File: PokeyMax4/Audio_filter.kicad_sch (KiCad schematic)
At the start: 16 parts, among them U1 TSV854IQ4T

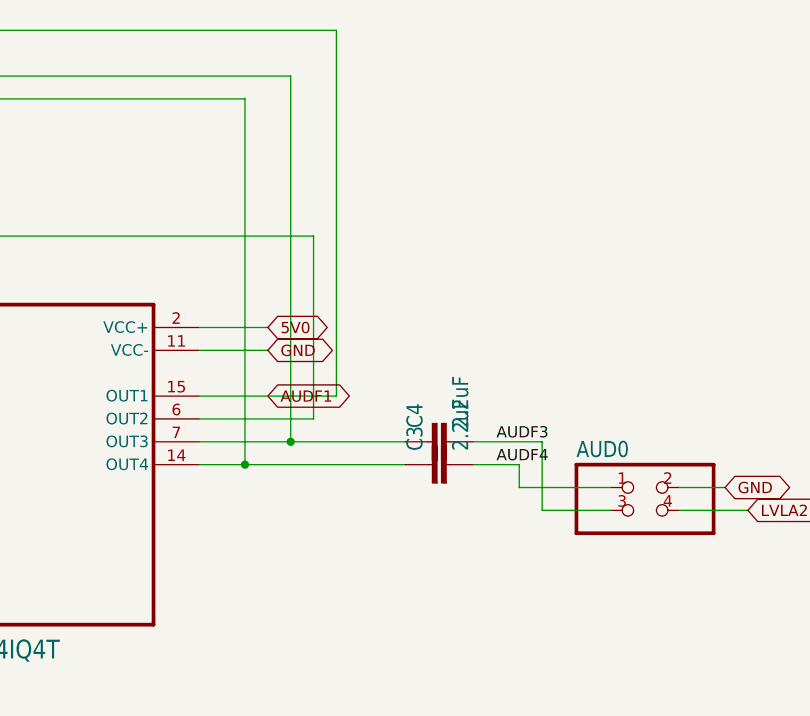
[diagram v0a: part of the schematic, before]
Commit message: Final adjustements to production files for JLC
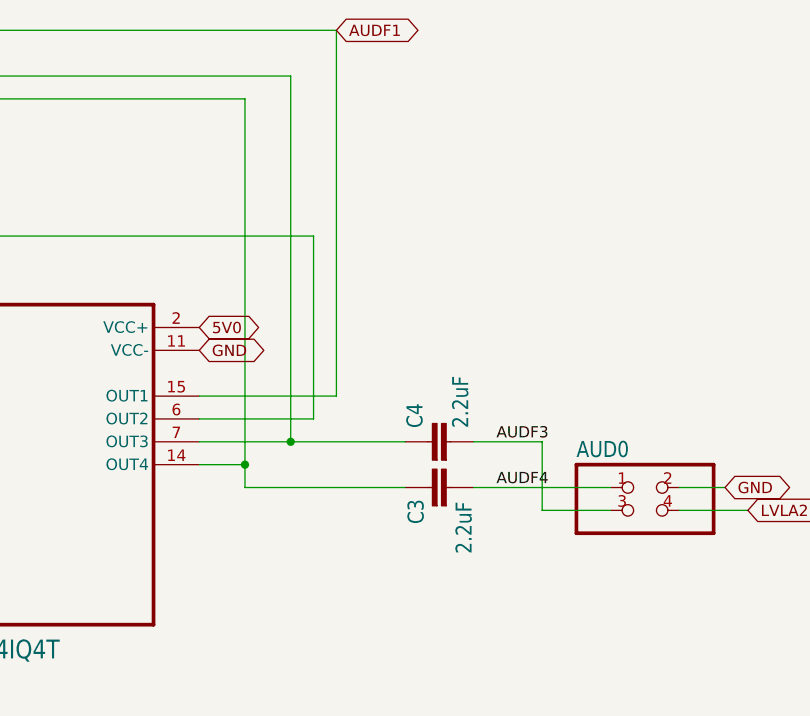
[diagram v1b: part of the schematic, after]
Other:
- moved on the sheet: C3
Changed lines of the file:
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@@
+	(wire
+		(pts
+			(xy 185.42 104.14) (xy 185.42 101.6)
+		)
+		(stroke
+			(width 0.1524)
+			(type solid)
+		)
+	)
 	(wire
 		(pts
@@
 	(wire
 		(pts
-			(xy 185.42 101.6) (xy 203.2 101.6)
+			(xy 185.42 104.14) (xy 203.2 104.14)
 		)
 		(stroke
@@
 	(wire
 		(pts
-			(xy 226.06 104.14) (xy 215.9 104.14)
-		)
-		(stroke
-			(width 0.1524)
-			(type solid)
-		)
-	)
-	(wire
-		(pts
 			(xy 68.58 99.06) (xy 68.58 109.22)
 		)
@@
 	(wire
 		(pts
-			(xy 180.34 88.9) (xy 187.96 88.9)
-		)
-		(stroke
-			(width 0.1524)
-			(type solid)
-		)
-	)
-	(wire
-		(pts
 			(xy 132.08 152.4) (xy 111.76 152.4)
 		)
@@
 	(wire
 		(pts
-			(xy 215.9 101.6) (xy 210.82 101.6)
+			(xy 210.82 104.14) (xy 226.06 104.14)
 		)
 		(stroke
@@
 	(wire
 		(pts
-			(xy 187.96 86.36) (xy 180.34 86.36)
-		)
-		(stroke
-			(width 0.1524)
-			(type solid)
-		)
-	)
-	(wire
-		(pts
 			(xy 101.6 142.24) (xy 132.08 142.24)
 		)
@@
 	(wire
 		(pts
-			(xy 215.9 104.14) (xy 215.9 101.6)
-		)
-		(stroke
-			(width 0.1524)
-			(type solid)
-		)
-	)
-	(wire
-		(pts
 			(xy 190.5 99.06) (xy 190.5 58.42)
 		)
@@
 	)
 	(label "AUDF4"
-		(at 213.36 101.6 0)
+		(at 213.36 104.14 0)
 		(fields_autoplaced yes)
 		(effects
@@
 	(global_label "5V0"
 		(shape bidirectional)
-		(at 187.96 86.36 0)
+		(at 180.34 86.36 0)
 		(fields_autoplaced yes)
 		(effects
@@
 		)
 		(property "Intersheetrefs" "${INTERSHEET_REFS}"
-			(at 195.4116 86.36 0)
+			(at 187.7916 86.36 0)
 			(effects
 				(font
@@
 	(global_label "GND"
 		(shape bidirectional)
-		(at 187.96 88.9 0)
+		(at 180.34 88.9 0)
 		(fields_autoplaced yes)
 		(effects
@@
 		)
 		(property "Intersheetrefs" "${INTERSHEET_REFS}"
-			(at 195.7673 88.9 0)
+			(at 188.1473 88.9 0)
 			(effects
 				(font
@@
 	(global_label "AUDF1"
 		(shape bidirectional)
-		(at 187.96 93.98 0)
+		(at 195.58 53.34 0)
 		(fields_autoplaced yes)
 		(effects
@@
 		)
 		(property "Intersheetrefs" "${INTERSHEET_REFS}"
-			(at 197.8416 93.98 0)
+			(at 205.4616 53.34 0)
 			(effects
 				(font
@@
 	(symbol
 		(lib_id "pokeymax4-eagle-import:C-EUC0402")
-		(at 205.74 101.6 90)
+		(at 205.74 104.14 90)
 		(unit 1)
 		(exclude_from_sim no)
@@
 		(dnp no)
 		(property "Reference" "C3"
-			(at 205.359 100.076 0)
+			(at 205.486 108.204 0)
 			(effects
 				(font
@@
 		)
 		(property "Value" "2.2uF"
-			(at 210.439 100.076 0)
+			(at 210.82 111.506 0)
 			(effects
 				(font
@@
 		)
 		(property "Footprint" "pokeymax4:C0402"
-			(at 205.74 101.6 0)
+			(at 205.74 104.14 0)
 			(effects
 				(font
@@
 		)
 		(property "Datasheet" ""
-			(at 205.74 101.6 0)
+			(at 205.74 104.14 0)
 			(effects
 				(font
@@
 		)
 		(property "Description" ""
-			(at 205.74 101.6 0)
+			(at 205.74 104.14 0)
 			(effects
 				(font
@@
 		)
 		(property "LCSC Part #" "C12530"
-			(at 205.74 101.6 0)
+			(at 205.74 104.14 0)
 			(effects
 				(font
@@
 		)
 		(property "JLCPCB Rotation Offset" ""
-			(at 205.74 101.6 0)
-			(effects
-				(font
+			(at 205.74 104.14 0)
+			(effects
+				(font
